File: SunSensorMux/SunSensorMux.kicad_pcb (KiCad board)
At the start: 2 copper layers, 44.3 x 89.9 mm, 7 parts, among them U1 TCA9548A_Multiplexer, U2 FEATHER_M0_BASIC_PROTO

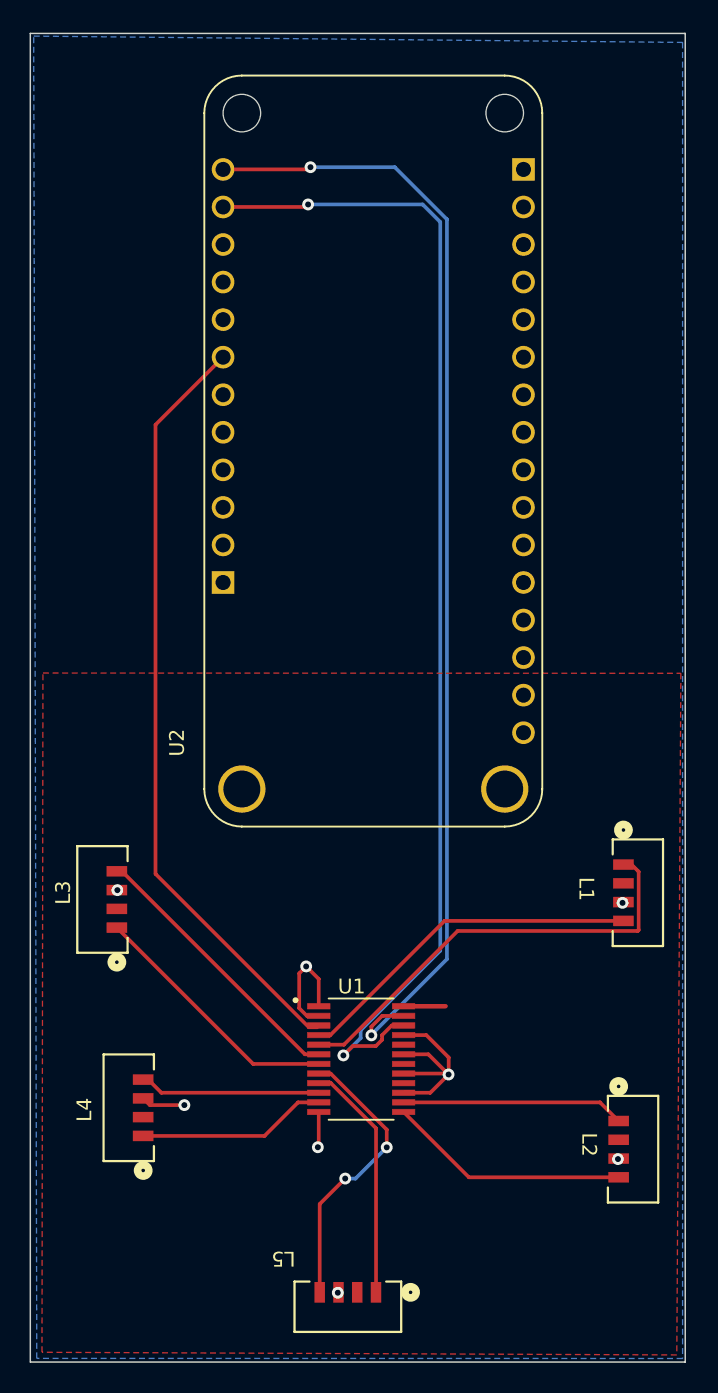
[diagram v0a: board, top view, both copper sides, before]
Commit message: Finish Routing
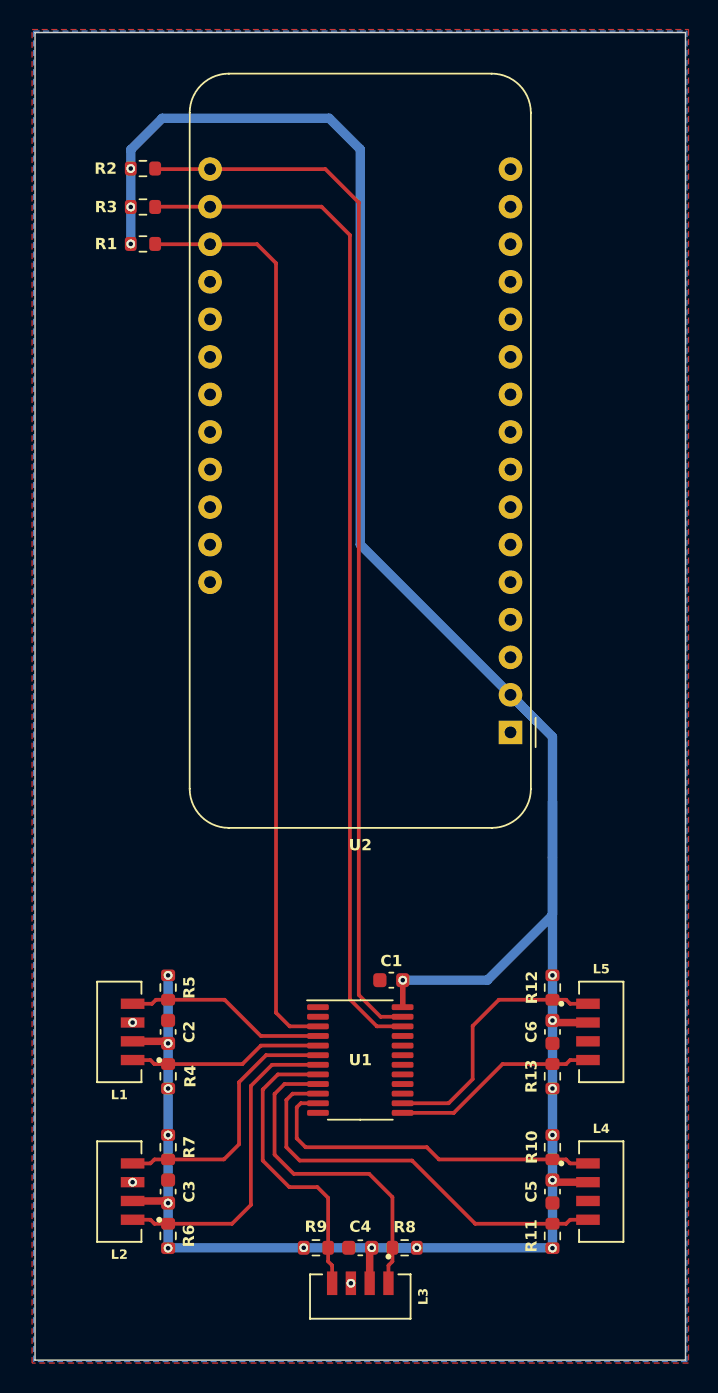
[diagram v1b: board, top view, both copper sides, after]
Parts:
- added C1: 1uF, Capacitor_SMD:C_0603_1608Metric, F.Cu at (192.0, 86.9)
- added C2: 0.1uF, Capacitor_SMD:C_0603_1608Metric, F.Cu at (176.9, 90.4)
- added C3: 0.1uF, Capacitor_SMD:C_0603_1608Metric, F.Cu at (176.9, 101.2)
- added C4: 0.1uF, Capacitor_SMD:C_0603_1608Metric, F.Cu at (189.9, 105.0)
- added C5: 0.1uF, Capacitor_SMD:C_0603_1608Metric, F.Cu at (202.9, 101.2)
- added C6: 0.1uF, Capacitor_SMD:C_0603_1608Metric, F.Cu at (202.9, 90.4)
- added R1: 10K, Resistor_SMD:R_0603_1608Metric, F.Cu at (175.2, 37.1)
- added R10: 10K, Resistor_SMD:R_0603_1608Metric, F.Cu at (202.9, 98.2)
- added R11: 10K, Resistor_SMD:R_0603_1608Metric, F.Cu at (202.9, 104.2)
- added R12: 10K, Resistor_SMD:R_0603_1608Metric, F.Cu at (202.9, 87.4)
- added R13: 10K, Resistor_SMD:R_0603_1608Metric, F.Cu at (202.9, 93.4)
- added R2: 10K, Resistor_SMD:R_0603_1608Metric, F.Cu at (175.2, 32.0)
- added R3: 10K, Resistor_SMD:R_0603_1608Metric, F.Cu at (175.2, 34.6)
- added R4: 10K, Resistor_SMD:R_0603_1608Metric, F.Cu at (176.9, 93.4)
- added R5: 10K, Resistor_SMD:R_0603_1608Metric, F.Cu at (176.9, 87.4)
- added R6: 10K, Resistor_SMD:R_0603_1608Metric, F.Cu at (176.9, 104.2)
- added R7: 10K, Resistor_SMD:R_0603_1608Metric, F.Cu at (176.9, 98.2)
- added R8: 10K, Resistor_SMD:R_0603_1608Metric, F.Cu at (192.9, 105.0)
- added R9: 10K, Resistor_SMD:R_0603_1608Metric, F.Cu at (186.9, 105.0)
- L1, L2, L3, L4, L5: footprint sunsensor:VEML7700-TR -> sunsensor:VEML7700-TT
- U1: footprint sunsensor:SOP65P640X120-24N -> Package_SO:TSSOP-24_4.4x7.8mm_P0.65mm
- U2: footprint sunsensor:MODULE_FEATHER_M0_BASIC_PROTO -> Module:Adafruit_Feather
- moved L1 36.3 mm to (173.6, 90.4), turned to 180 degrees
- moved L2 34.9 mm to (173.6, 101.2), turned to 180 degrees
- moved L4 32.5 mm to (206.2, 101.2), turned to 0 degrees
- moved L3 32.0 mm to (189.9, 108.3), turned to -90 degrees
- moved L5 25.3 mm to (206.2, 90.4), turned to 0 degrees
- moved U2 21.2 mm to (200.1, 70.1), turned to 180 degrees
- moved U1 0.08 mm to (189.9, 92.3)
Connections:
- L1 pad 2: +3V3 -> +3.3V
- L2 pad 1: /SCL4 -> /SCL1
- L2 pad 2: +3V3 -> +3.3V
- L2 pad 4: /SDA4 -> /SDA1
- L3 pad 1: /SCL1 -> /SCL2
- L3 pad 2: +3V3 -> +3.3V
- L3 pad 4: /SDA1 -> /SDA2
- L4 pad 2: +3V3 -> +3.3V
- L5 pad 1: Net-(L5-Pad1) -> /SCL4
- L5 pad 2: +3V3 -> +3.3V
- L5 pad 4: /SDA2 -> /SDA4
- U1 pad 15: GND -> /SDA5
- U1 pad 16: unconnected-(U1-Pad16) -> /SCL5
- U1 pad 17: GND -> /SDA6
- U1 pad 18: unconnected-(U1-Pad18) -> /SCL6
- U1 pad 19: GND -> /SDA7
- U1 pad 20: unconnected-(U1-Pad20) -> /SCL7
- U1 pad 24: +3V3 -> +3.3V
- U1 pad 9: Net-(L5-Pad1) -> /SCL2
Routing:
- net +3.3V: track 0.00 -> 187.9 mm, vias 0 -> 19
- net GND: track 28.1 -> 0.00 mm, vias 8 -> 3
- net /SCL2: track 0.00 -> 22.4 mm
- net /SCL0: track 30.0 -> 13.2 mm
- net Net-(L5-Pad1): track 16.2 -> 0.00 mm
- net /SDA3: track 12.2 -> 28.2 mm
- net /SCL3: track 12.8 -> 24.1 mm
- net /RESET: track 52.2 -> 62.6 mm
- net /SDA0: track 23.8 -> 13.7 mm
- net /SCL: track 79.4 -> 70.0 mm, vias 2 -> 0
- net /SDA: track 77.0 -> 71.9 mm, vias 2 -> 0
- net /SCL1: track 17.5 -> 21.8 mm
- net +3V3: track 2.84 -> 0.00 mm
- net /SCL4: track 15.1 -> 17.7 mm
- net /SDA4: track 16.4 -> 14.0 mm
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- added copper zone on F.Cu, net GND
- removed copper zone on F.Cu, net +3V3
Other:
- board size 44.3 x 89.9 mm -> 44 x 89.8 mm
